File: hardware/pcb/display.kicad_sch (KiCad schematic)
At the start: 9 parts, among them J8 503480-1000

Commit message: added lcsc part nr to display conn
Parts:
- J8: LCSC (none) -> C127355
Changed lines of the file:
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@@
+			)
+		)
+		(property "LCSC" "C127355"
+			(at 130.81 69.85 0)
+			(hide yes)
+			(show_name no)
+			(do_not_autoplace no)
+			(effects
+				(font
+					(size 1.27 1.27)
+				)
 			)
 		)

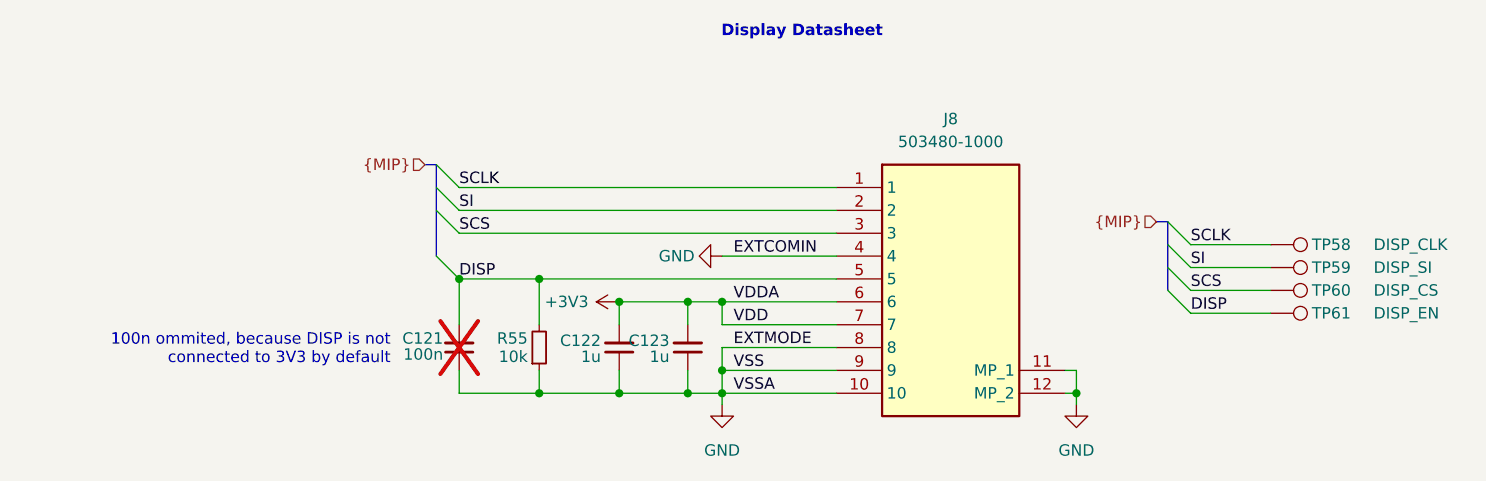
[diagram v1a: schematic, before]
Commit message: cleanup, tespoints, passives
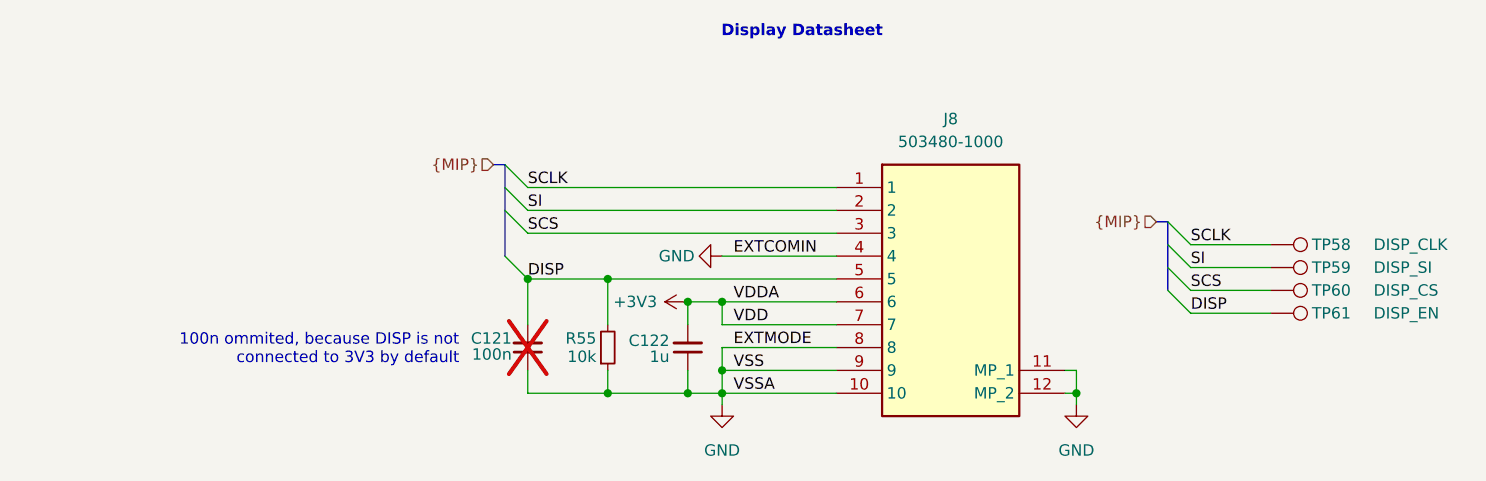
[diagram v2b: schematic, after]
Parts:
- removed C123: 1u, Capacitor_SMD:C_0402_1005Metric, symbol Device:C_Small
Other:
- moved on the sheet: C121, C122, R55
